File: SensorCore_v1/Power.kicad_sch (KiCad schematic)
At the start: 18 parts, among them U3 R-78C5.0-1.0, U5 R-78K3.3-1.0

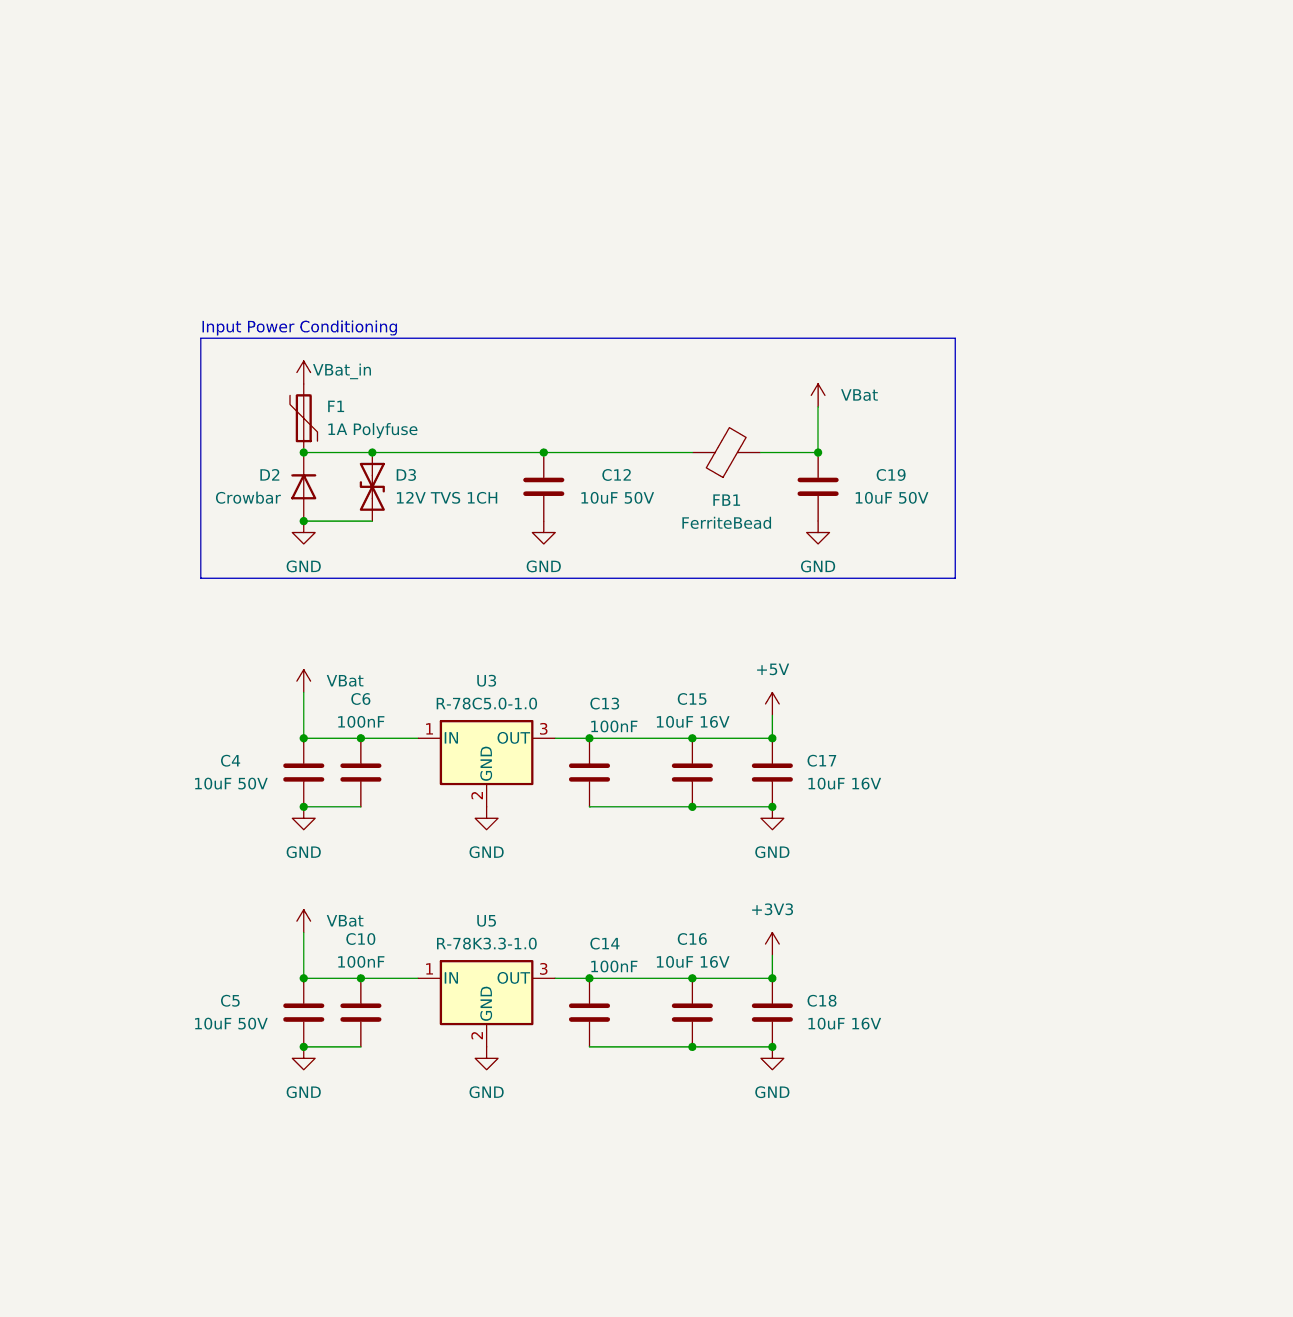
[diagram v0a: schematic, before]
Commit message: Preliminary design done
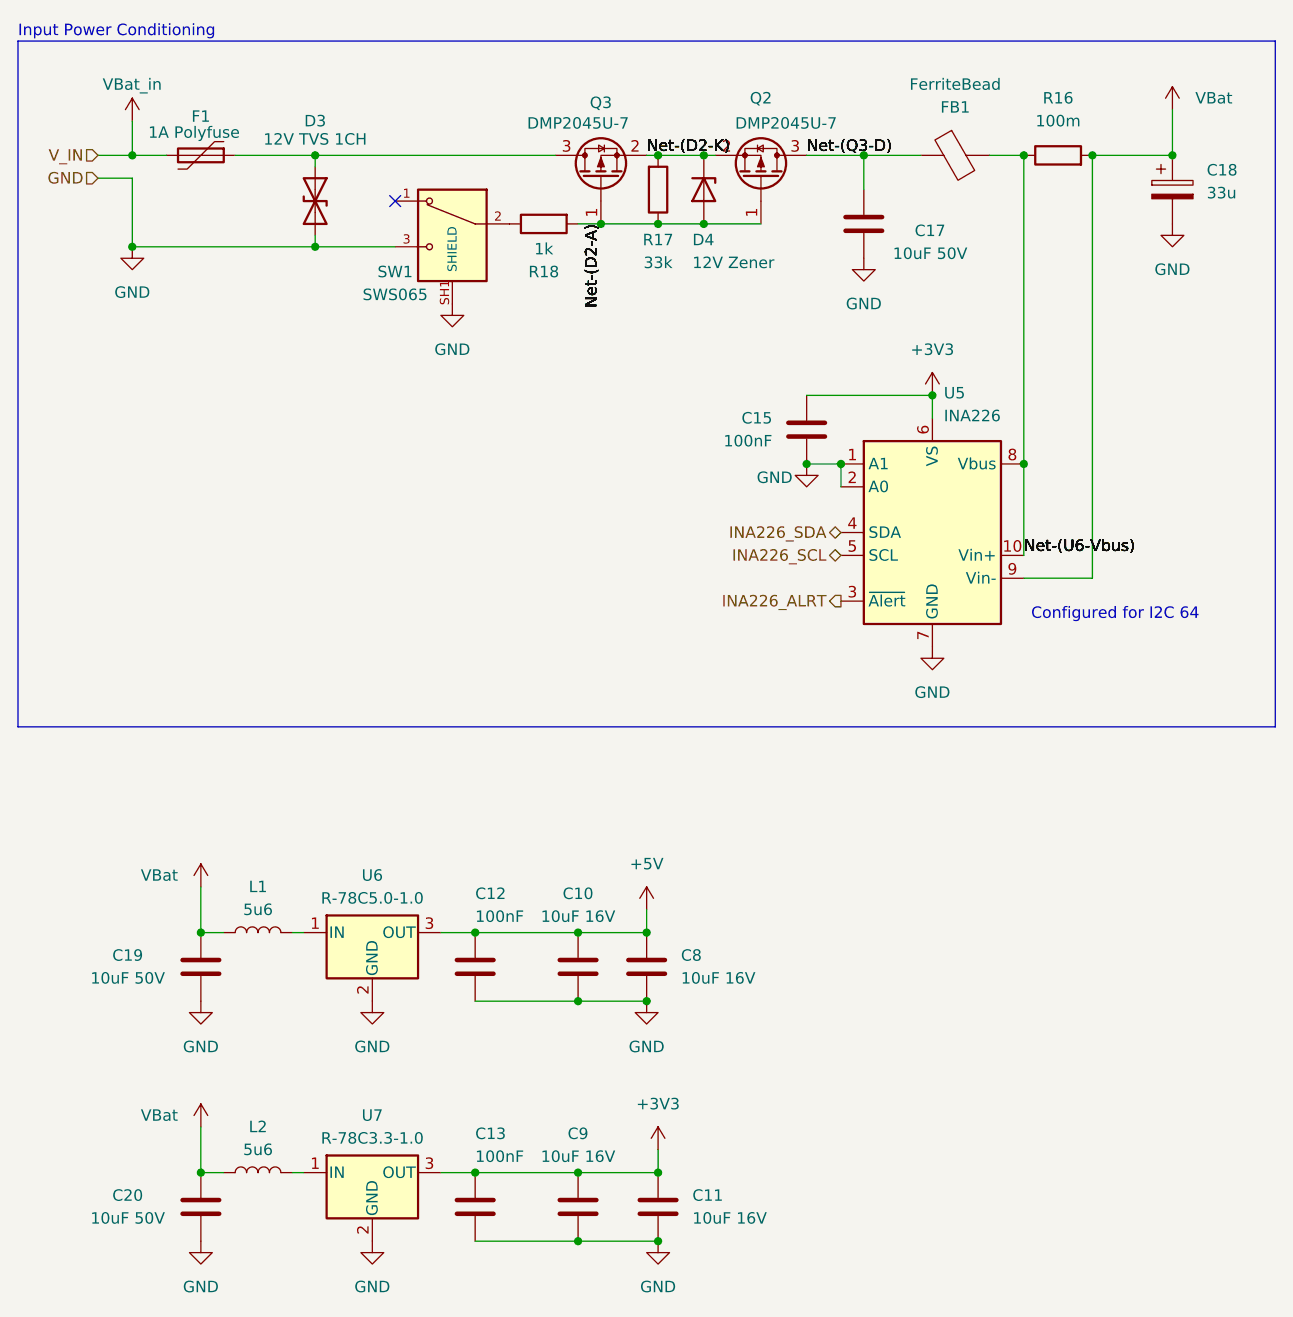
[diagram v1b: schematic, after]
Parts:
- removed C10, C6: 100nF, Resistor_SMD:R_0603_1608Metric_Pad0.98x0.95mm_HandSolder, symbol Device:C
- removed C19: 10uF 50V, Capacitor_SMD:C_0805_2012Metric_Pad1.18x1.45mm_HandSolder, symbol Device:C
- removed D2: Crowbar, symbol Device:D
- removed D3: 12V TVS 1CH, Diode_SMD:D_SMA, symbol Device:D_TVS
- removed F1: 1A Polyfuse, Resistor_SMD:R_1206_3216Metric_Pad1.30x1.75mm_HandSolder, symbol Device:Polyfuse
- added C15: 100nF, Capstone Footprints:C_0603_1608Metric_Pad1.08x0.95mm_HandSolder, symbol Project:C
- added C18: 33u, Capstone Footprints:CP_Radial_D6.3mm_P2.50mm, symbol Device:C_Polarized
- added D3: 12V TVS 1CH, Capstone Footprints:D_SMA, symbol Project:D_TVS
- added D4: 12V Zener, Capstone Footprints:D_SOD-123, symbol Device:D_Zener
- added F1: 1A Polyfuse, Capstone Footprints:R_1206_3216Metric_Pad1.30x1.75mm_HandSolder, symbol Project:Polyfuse
- added L1, L2: 5u6, Capstone Footprints:IFSC2020DEER5R6M01, symbol Device:L
- added Q2, Q3: DMP2045U-7, Capstone Footprints:SOT-23-3, symbol Project:Q_PMOS_GSD
- added R16: 100m, Capstone Footprints:R_0805_2012Metric_Pad1.20x1.40mm_HandSolder, symbol Project:R
- added R17: 33k, Capstone Footprints:R_0603_1608Metric_Pad0.98x0.95mm_HandSolder, symbol Project:R
- added R18: 1k, Capstone Footprints:R_0603_1608Metric_Pad0.98x0.95mm_HandSolder, symbol Project:R
- added SW1: SWS065, Capstone Footprints:SW_SWS065-030V12TSK_REVA, symbol Project:SWS065-030V12TSK_REVA
- added U5: INA226, Capstone Footprints:TSSOP-10_3x3mm_P0.5mm, symbol Project:INA226
- C10: renamed from C15; footprint Capacitor_SMD:C_0805_2012Metric_Pad1.18x1.45mm_HandSolder -> Capstone Footprints:C_0805_2012Metric_Pad1.18x1.45mm_HandSolder; symbol Device:C -> Project:C; KiLib_Generator (none) -> SMD_2terminal_chip_molded
- C11: renamed from C18; footprint Capacitor_SMD:C_0805_2012Metric_Pad1.18x1.45mm_HandSolder -> Capstone Footprints:C_0805_2012Metric_Pad1.18x1.45mm_HandSolder; symbol Device:C -> Project:C; KiLib_Generator (none) -> SMD_2terminal_chip_molded
- C12: renamed from C13; footprint Resistor_SMD:R_0603_1608Metric_Pad0.98x0.95mm_HandSolder -> Capstone Footprints:C_0603_1608Metric_Pad1.08x0.95mm_HandSolder; symbol Device:C -> Project:C; KiLib_Generator (none) -> SMD_2terminal_chip_molded
- C13: renamed from C14; footprint Resistor_SMD:R_0603_1608Metric_Pad0.98x0.95mm_HandSolder -> Capstone Footprints:C_0603_1608Metric_Pad1.08x0.95mm_HandSolder; symbol Device:C -> Project:C; KiLib_Generator (none) -> SMD_2terminal_chip_molded
- C17: renamed from C12; footprint Capacitor_SMD:C_0805_2012Metric_Pad1.18x1.45mm_HandSolder -> Capstone Footprints:C_0805_2012Metric_Pad1.18x1.45mm_HandSolder; symbol Device:C -> Project:C; KiLib_Generator (none) -> SMD_2terminal_chip_molded
- C19: renamed from C4; footprint Capacitor_SMD:C_0805_2012Metric_Pad1.18x1.45mm_HandSolder -> Capstone Footprints:C_0805_2012Metric_Pad1.18x1.45mm_HandSolder; symbol Device:C -> Project:C; KiLib_Generator (none) -> SMD_2terminal_chip_molded
- C20: renamed from C5; footprint Capacitor_SMD:C_0805_2012Metric_Pad1.18x1.45mm_HandSolder -> Capstone Footprints:C_0805_2012Metric_Pad1.18x1.45mm_HandSolder; symbol Device:C -> Project:C; KiLib_Generator (none) -> SMD_2terminal_chip_molded
- C8: renamed from C17; footprint Capacitor_SMD:C_0805_2012Metric_Pad1.18x1.45mm_HandSolder -> Capstone Footprints:C_0805_2012Metric_Pad1.18x1.45mm_HandSolder; symbol Device:C -> Project:C; KiLib_Generator (none) -> SMD_2terminal_chip_molded
- C9: renamed from C16; footprint Capacitor_SMD:C_0805_2012Metric_Pad1.18x1.45mm_HandSolder -> Capstone Footprints:C_0805_2012Metric_Pad1.18x1.45mm_HandSolder; symbol Device:C -> Project:C; KiLib_Generator (none) -> SMD_2terminal_chip_molded
- FB1: footprint Resistor_SMD:R_0603_1608Metric_Pad0.98x0.95mm_HandSolder -> Capstone Footprints:R_0603_1608Metric_Pad0.98x0.95mm_HandSolder; symbol Device:FerriteBead -> Project:FerriteBead; KiLib_Generator (none) -> SMD_2terminal_chip_molded
- U6: renamed from U3; footprint Converter_DCDC:Converter_DCDC_RECOM_R-78E-0.5_THT -> Capstone Footprints:Converter_DCDC_RECOM_R-78E-0.5_THT; symbol Regulator_Switching:R-78C5.0-1.0 -> Project:R-78C5.0-1.0; KiLib_Generator (none) -> Recom_DCDC
- U7: renamed from U5; value R-78K3.3-1.0 -> R-78C3.3-1.0; footprint Converter_DCDC:Converter_DCDC_RECOM_R-78B-2.0_THT -> Capstone Footprints:Converter_DCDC_RECOM_R-78E-0.5_THT; symbol Regulator_Switching:R-78B1.2-2.0 -> Project:R-78B1.2-2.0; KiLib_Generator (none) -> Recom_DCDC
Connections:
- net +3V3: now also C15.2, U5.6 (VS)
- net GND: now also C15.1, C18.2, D3.2 (A2), SW1.3, SW1.SH1 (SHIELD), SW1.SH2 (SHIELD__1), U5.1 (A1), U5.2 (A0), U5.7 (GND)
- net VBat: now also C18.1, L1.1, L2.1, R16.2, U5.9 (Vin-); no longer FB1.2, U6.1 (IN), U7.1 (IN)
- net VBat_in: now also F1.2
- net Net-(Q3-D): now reaches C17.1, FB1.1
- net Net-(Q3-D): now also Q2.3 (D)
- new net: R18.1, SW1.2
- new net: D3.1 (A1), F1.1, Q3.3 (D)
- new net: L2.2, U7.1 (IN)
- new net: L1.2, U6.1 (IN)
- new net INA226_ALRT: U5.3 (~{Alert})
- new net INA226_SCL: U5.5 (SCL)
- new net INA226_SDA: U5.4 (SDA)
- new net Net-(D2-A): D4.2 (A), Q2.1 (G), Q3.1 (G), R17.1, R18.2
- new net Net-(D2-K): D4.1 (K), Q2.2 (S), Q3.2 (S), R17.2
- new net Net-(U6-Vbus): FB1.2, R16.1, U5.10 (Vin+), U5.8 (Vbus)
- no-connect marks 0 -> 1
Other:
- note added: "Configured for I2C 64"
- moved on the sheet: C10, C11, C12, C13, C17, C19, C20, C8, C9, FB1, U6, U7
